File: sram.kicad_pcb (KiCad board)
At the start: 4 copper layers, 97.2 x 28.2 mm, 25 parts, among them J1 Cache_slot, M1 UM61256AS, M2 UM61256AS, M3 UM61256AS, M4 UM61256AS, M5 UM61256AS, M6 UM61256AS, M7 UM61256AS, M8 UM61256AS, U1 74F244, U2 74F244

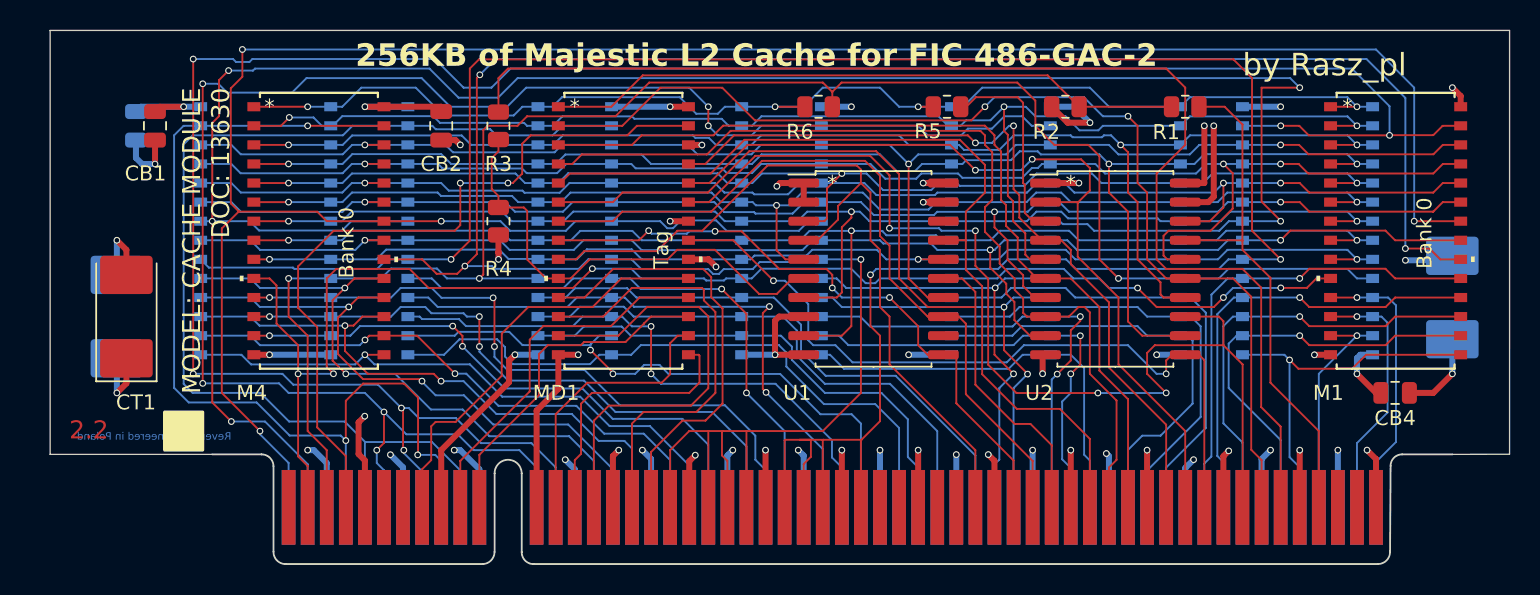
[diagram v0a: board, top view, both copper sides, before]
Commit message: Final Rev 2.3
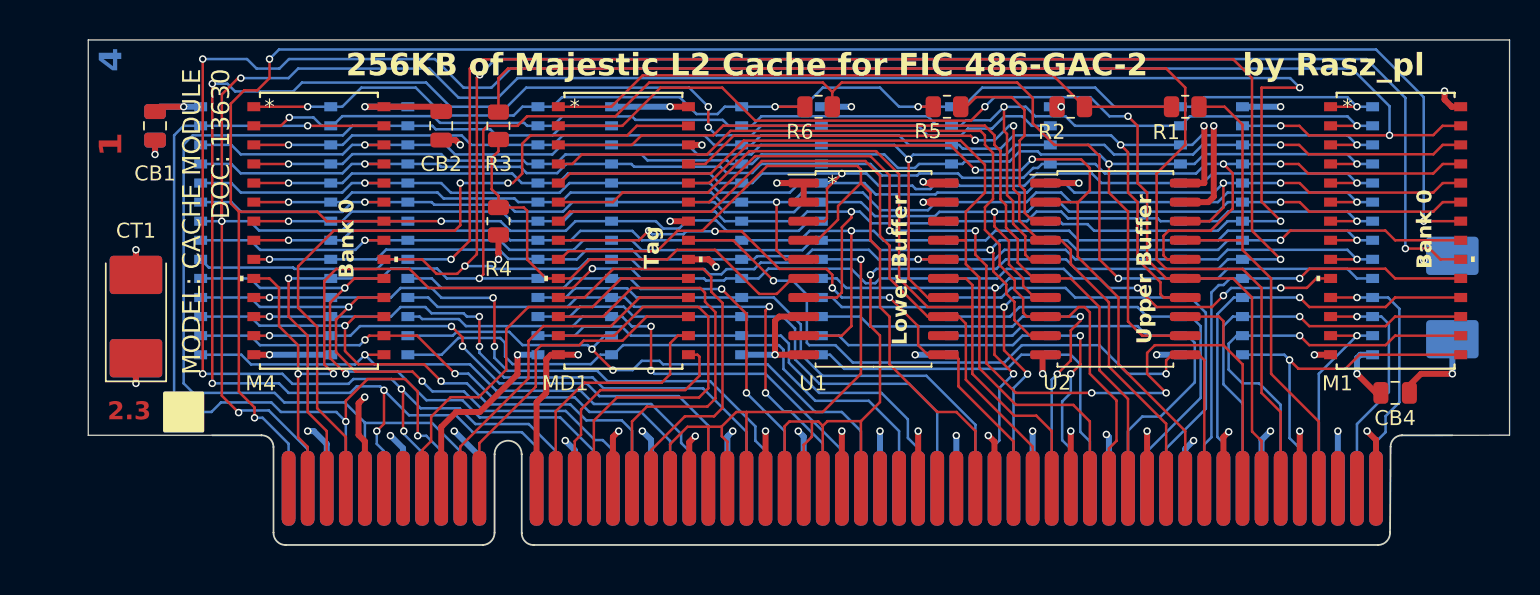
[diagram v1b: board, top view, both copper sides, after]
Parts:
- moved CB3 1.27 mm to (125.7, 83.8)
- moved CT2 1.27 mm to (124.5, 96.5)
- moved J1 1.27 mm to (171.4, 108.0)
- moved CT1 0.63 mm to (124.5, 96.5)
- moved R2 0.36 mm to (186.7, 82.5)
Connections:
- J1 pad b43: +5V -> GND
- J1 pad b48: GND -> +5V
- J1 pad b52: +5V -> GND
- J1 pad b56: GND -> +5V
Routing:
- net GND: track 154.5 -> 145.5 mm
- net +5V: track 82.7 -> 77.3 mm
- net Bank0_CS: track 166.2 -> 162.4 mm
- net Bank0_OE: track 164.9 -> 161.7 mm
- net Bank1_CS: track 160.2 -> 157.8 mm
- net Byte_WE3: track 65.3 -> 63.1 mm
- net TAG_Q3: track 18.1 -> 16.3 mm
- net CPU_D20: track 40.8 -> 39.0 mm
- net Byte_WE1: track 115.7 -> 114.2 mm
- net CPU_D21: track 38.8 -> 37.4 mm
- net CPU_A11: track 53.5 -> 52.1 mm
- net CPU_A5: track 43.4 -> 42.1 mm
- net CPU_A12: track 57.1 -> 55.8 mm
- net CPU_A15: track 73.4 -> 72.1 mm
- net CPU_A6: track 51.0 -> 49.7 mm
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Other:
- board size 97.2 x 28.2 mm -> 94.6 x 26.3 mm
- board text added: "1"
- board text added: "2"
- board text added: "2.3"
- board text added: "3"
- board text added: "4"
- board text added: "Lower Buffer"
- board text added: "Reverse Engineered in Poland"
- board text added: "Upper Buffer"
- board text removed: "2.2"
- board text removed: "Reverse engineered in Poland"
